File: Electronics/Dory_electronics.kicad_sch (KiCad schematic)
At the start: 22 parts, among them J1 Bateria 2S, J10 SHARP_CENTRO_E, J4 Motor B, J5 Motor A, J6 sensor IR, J7 VL53L0X_ESQUERDO, J8 SHARP_CENTRO_D, J9 VL53L0X_DIREITO, U1 LM1117 5V

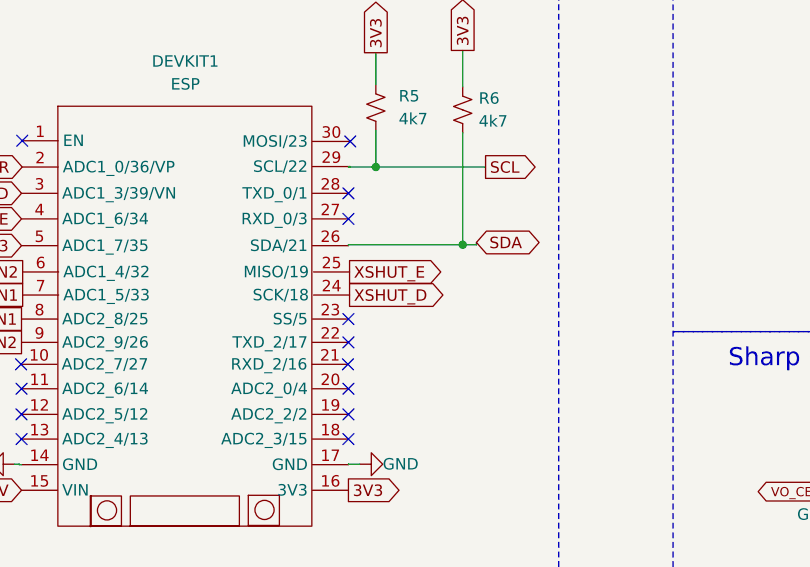
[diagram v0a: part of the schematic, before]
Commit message: chore: update schematic and PCB
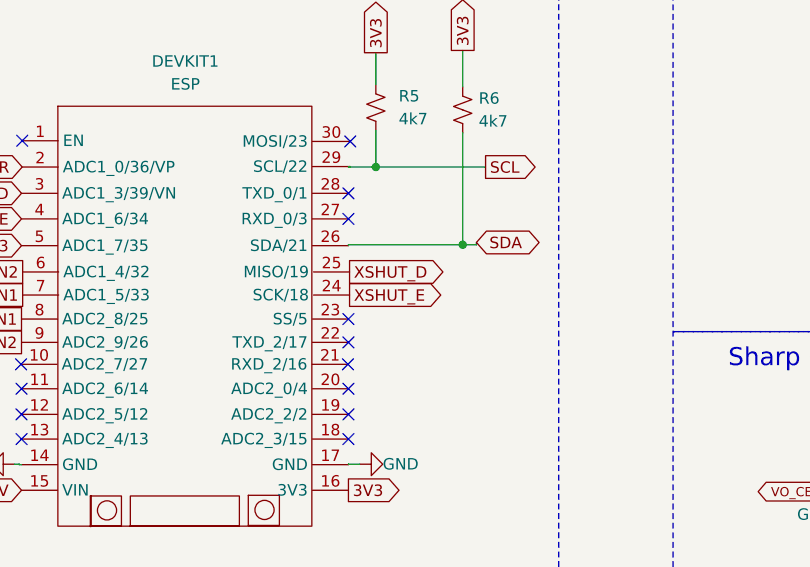
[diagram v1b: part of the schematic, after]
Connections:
- net XSHUT_D: now also DEVKIT1.25 (MISO/19); no longer DEVKIT1.24 (SCK/18)
- net XSHUT_E: now also DEVKIT1.24 (SCK/18); no longer DEVKIT1.25 (MISO/19)
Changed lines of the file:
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@@
+	)
+	(no_connect
+		(at 71.12 67.31)
 	)
 	(no_connect
@@
 	)
 	(no_connect
+		(at 43.18 67.31)
+	)
+	(no_connect
 		(at 162.052 108.2548)
 	)
@@
 	(no_connect
 		(at 162.0012 102.6922)
-	)
-	(no_connect
-		(at 43.18 67.31)
-	)
-	(no_connect
-		(at 71.12 67.31)
 	)
 	(no_connect
@@
 		)
 	)
+	(global_label "XSHUT_E"
+		(shape output)
+		(at 162.179 94.996 0)
+		(effects
+			(font
+				(size 1.27 1.27)
+			)
+			(justify left)
+		)
+		(property "Intersheetrefs" "${INTERSHEET_REFS}"
+			(at 162.179 94.996 0)
+			(effects
+				(font
+					(size 1.27 1.27)
+				)
+				(hide yes)
+			)
+		)
+	)
+	(global_label "BIN1"
+		(shape output)
+		(at 125.857 94.996 180)
+		(effects
+			(font
+				(size 1.27 1.27)
+			)
+			(justify right)
+		)
+		(property "Intersheetrefs" "${INTERSHEET_REFS}"
+			(at 125.857 94.996 0)
+			(effects
+				(font
+					(size 1.27 1.27)
+				)
+				(hide yes)
+			)
+		)
+	)
+	(global_label "BO2"
+		(shape input)
+		(at 66.167 32.766 90)
+		(fields_autoplaced yes)
+		(effects
+			(font
+				(size 1.016 1.016)
+			)
+			(justify left)
+		)
+		(property "Intersheetrefs" "${INTERSHEET_REFS}"
+			(at 66.167 27.3301 90)
+			(effects
+				(font
+					(size 1.27 1.27)
+				)
+				(justify left)
+				(hide yes)
+			)
+		)
+	)
+	(global_label "2S"
+		(shape input)
+		(at 55.88 147.32 90)
+		(fields_autoplaced yes)
+		(effects
+			(font
+				(size 1.27 1.27)
+			)
+			(justify left)
+		)
+		(property "Intersheetrefs" "${INTERSHEET_REFS}"
+			(at 55.88 141.9158 90)
+			(effects
+				(font
+					(size 1.27 1.27)
+				)
+				(justify left)
+				(hide yes)
+			)
+		)
+	)
+	(global_label "SCL"
+		(shape input)
+		(at 237.49 71.12 180)
+		(effects
+			(font
+				(size 1.27 1.27)
+			)
+			(justify right)
+		)
+		(property "Intersheetrefs" "${INTERSHEET_REFS}"
+			(at 237.49 71.12 0)
+			(effects
+				(font
+					(size 1.27 1.27)
+				)
+				(hide yes)
+			)
+		)
+	)
 	(global_label "XSHUT_D"
 		(shape output)
-		(at 162.179 94.996 0)
-		(effects
-			(font
-				(size 1.27 1.27)
-			)
-			(justify left)
-		)
-		(property "Intersheetrefs" "${INTERSHEET_REFS}"
-			(at 162.179 94.996 0)
-			(effects
-				(font
-					(size 1.27 1.27)
-				)
-				(hide yes)
-			)
-		)
-	)
-	(global_label "BIN1"
-		(shape output)
-		(at 125.857 94.996 180)
-		(effects
-			(font
-				(size 1.27 1.27)
-			)
-			(justify right)
-		)
-		(property "Intersheetrefs" "${INTERSHEET_REFS}"
-			(at 125.857 94.996 0)
-			(effects
-				(font
-					(size 1.27 1.27)
-				)
-				(hide yes)
-			)
-		)
-	)
-	(global_label "BO2"
-		(shape input)
-		(at 66.167 32.766 90)
-		(fields_autoplaced yes)
-		(effects
-			(font
-				(size 1.016 1.016)
-			)
-			(justify left)
-		)
-		(property "Intersheetrefs" "${INTERSHEET_REFS}"
-			(at 66.167 27.3301 90)
-			(effects
-				(font
-					(size 1.27 1.27)
-				)
-				(justify left)
-				(hide yes)
-			)
-		)
-	)
-	(global_label "2S"
-		(shape input)
-		(at 55.88 147.32 90)
-		(fields_autoplaced yes)
-		(effects
-			(font
-				(size 1.27 1.27)
-			)
-			(justify left)
-		)
-		(property "Intersheetrefs" "${INTERSHEET_REFS}"
-			(at 55.88 141.9158 90)
-			(effects
-				(font
-					(size 1.27 1.27)
-				)
-				(justify left)
-				(hide yes)
-			)
-		)
-	)
-	(global_label "SCL"
-		(shape input)
-		(at 237.49 71.12 180)
-		(effects
-			(font
-				(size 1.27 1.27)
-			)
-			(justify right)
-		)
-		(property "Intersheetrefs" "${INTERSHEET_REFS}"
-			(at 237.49 71.12 0)
-			(effects
-				(font
-					(size 1.27 1.27)
-				)
-				(hide yes)
-			)
-		)
-	)
-	(global_label "XSHUT_E"
-		(shape output)
 		(at 162.179 92.4306 0)
